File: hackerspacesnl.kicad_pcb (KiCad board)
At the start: 2 copper layers, 82.7 x 99.6 mm, 53 parts, among them J1 Screw_Terminal_01x02, J2 Conn_01x04_Male, Q1 Q_NMOS_GSD, Q2 Q_NMOS_GSD, Q3 Q_NMOS_GSD, Q4 Q_NMOS_GSD, Q5 Q_NMOS_GSD, Q6 Q_NMOS_GSD, SW1 SW_Push, SW2 SW_Push, U1 AMS1117-3.3, U2 ESP32-wroom-32

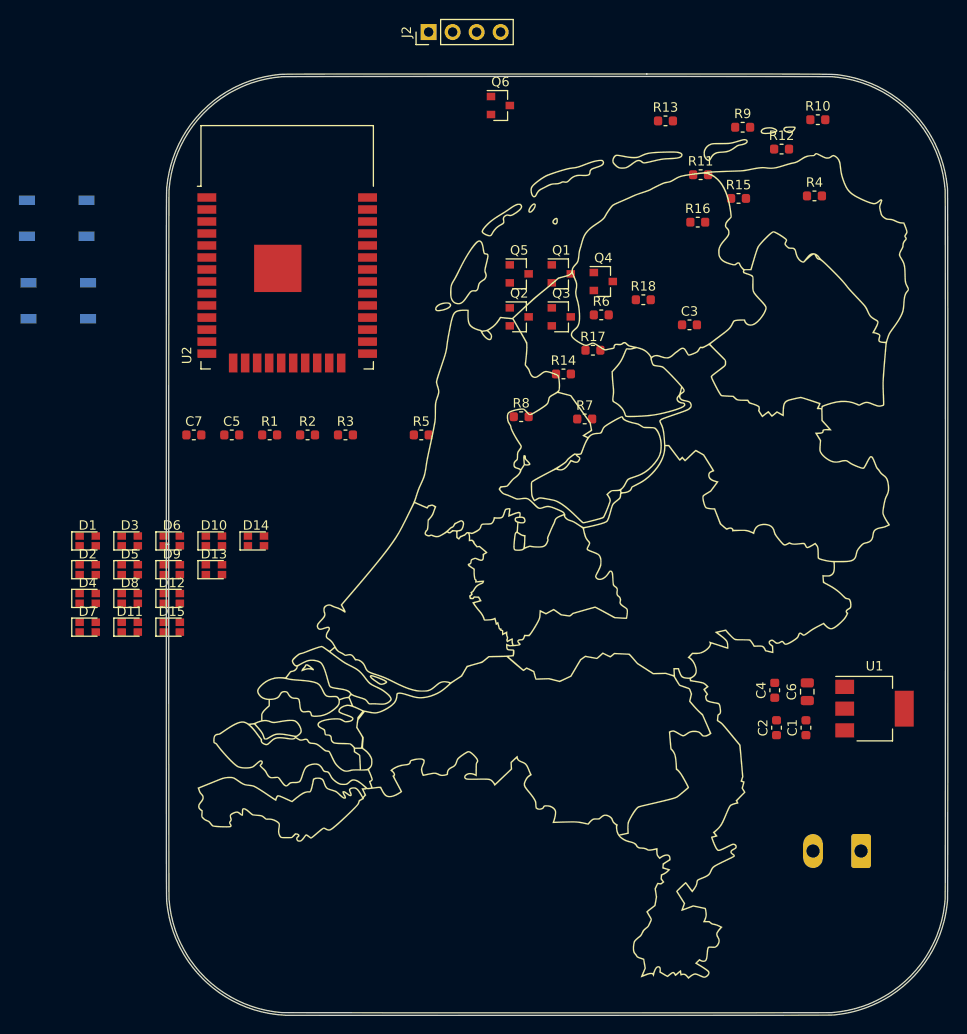
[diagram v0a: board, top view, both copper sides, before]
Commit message: board outline
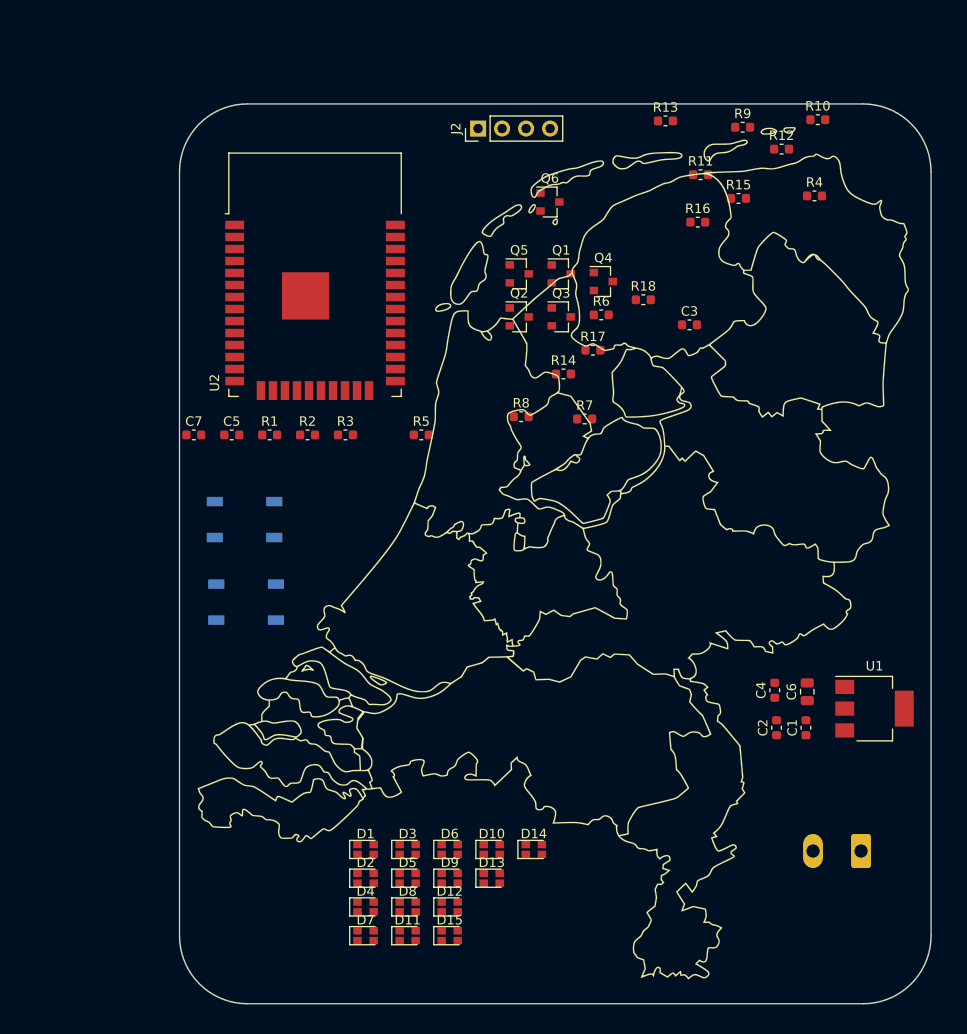
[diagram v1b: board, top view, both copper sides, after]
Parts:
- moved D5 43.9 mm to (100.5, 126.4)
- moved D9 43.9 mm to (104.9, 126.4)
- moved D12 43.9 mm to (104.9, 129.5)
- moved D3 43.9 mm to (100.5, 123.4)
- moved D6 43.9 mm to (104.9, 123.4)
- moved D8 43.9 mm to (100.5, 129.5)
- moved D13 43.9 mm to (109.4, 126.4)
- moved D2 43.9 mm to (96.0, 126.4)
- moved D1 43.9 mm to (96.0, 123.4)
- moved D10 43.9 mm to (109.4, 123.4)
- moved D11 43.9 mm to (100.5, 132.5)
- moved D14 43.9 mm to (113.8, 123.4)
- moved D15 43.9 mm to (104.9, 132.5)
- moved D4 43.9 mm to (96.0, 129.5)
- moved D7 43.9 mm to (96.0, 132.5)
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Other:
- board size 82.7 x 99.6 mm -> 79.5 x 95.2 mm
